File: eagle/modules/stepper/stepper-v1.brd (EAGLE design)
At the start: 100 x 80 mm, 11 parts, among them J1 RJ12RIGHTANGLE

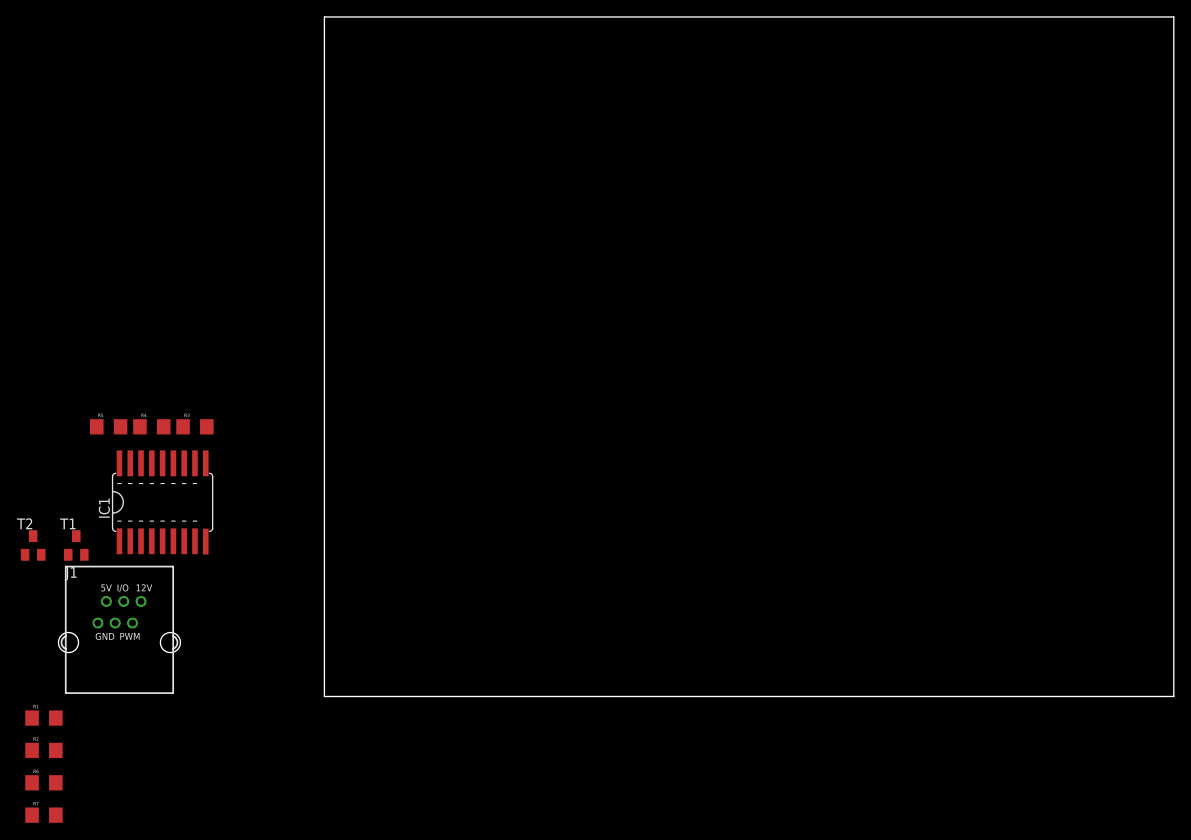
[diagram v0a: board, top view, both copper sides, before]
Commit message: Update Stepper
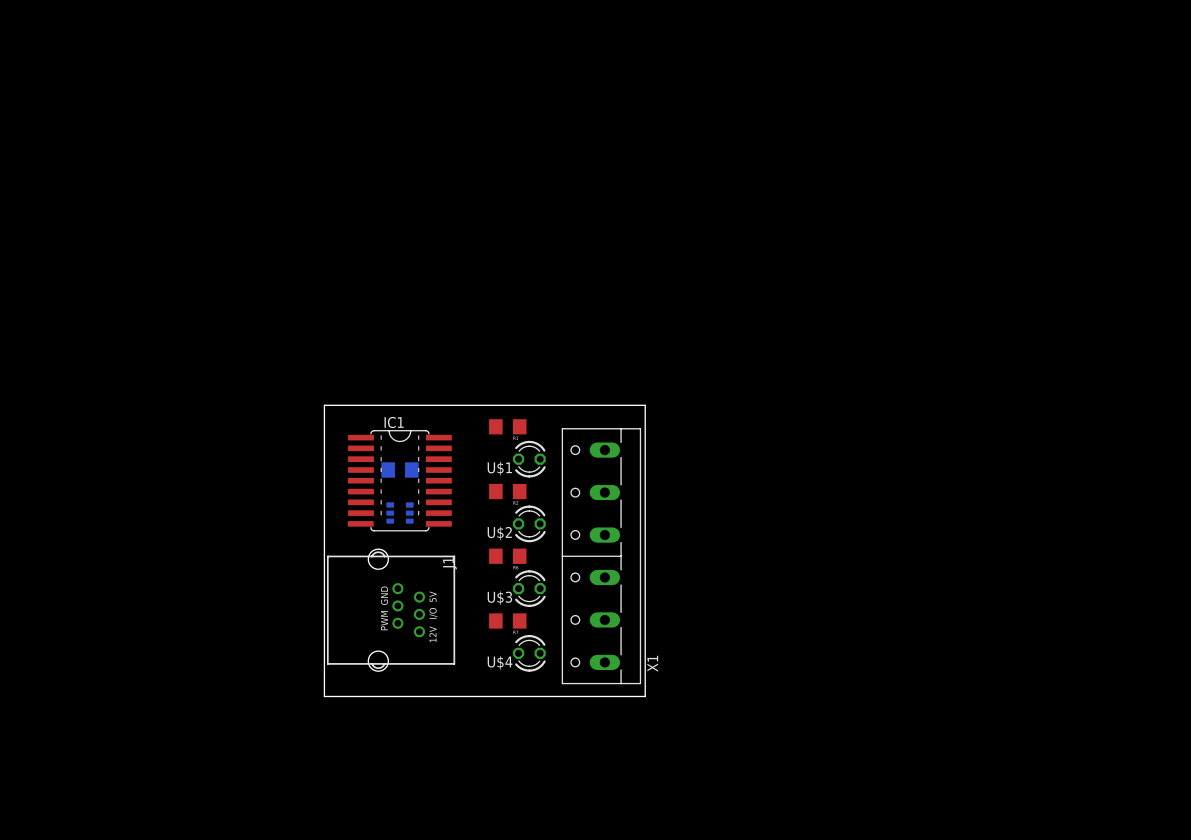
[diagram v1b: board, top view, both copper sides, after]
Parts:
- removed R3, R4: 1k, SparkFun:1206
- removed T1, T2: (no value), transistor:SOT23-BEC
- added IC2: SN74LVC2G14, lpatiny:SOT23-6
- added U$1, U$2, U$3, U$4: LED3MM, lpatiny:LED3MM
- added X1: (no value), con-wago-500:W237-6
- moved R1 64.5 mm to (21.6, 31.8), turned to 180 degrees
- moved R2 62.5 mm to (21.6, 24.1), turned to 180 degrees
- moved R6 60.8 mm to (21.6, 16.5), turned to 180 degrees
- moved R7 59.2 mm to (21.6, 8.89), turned to 180 degrees
- moved R5 34.7 mm to (8.89, 26.7), flipped to the bottom, turned to 180 degrees
- moved J1 30.7 mm to (6.35, 10.2), turned to 270 degrees
- moved IC1 28.1 mm to (8.89, 25.4), turned to 270 degrees
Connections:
- removed net N$15: IC1.7, IC1.8, R4.2, T2.C
- new net N$10: R2.1, U$2.K
- new net N$11: R6.1, U$3.K
- new net N$12: R7.1, U$4.K
- new net N$7: IC1.7, IC1.8, IC2.4
- new net N$9: R1.1, U$1.K
- net +12V: now also X1.2, X1.5
- net +5V: now also IC2.5, U$1.A, U$2.A, U$3.A, U$4.A; no longer R3.1, R4.1
- net GND: now also IC2.2; no longer T1.E, T2.E
- net N$1: now also IC2.1; no longer T1.B
- net N$14: now also IC1.5, IC1.6, IC2.6; no longer IC1.3, IC1.4, R3.2, T1.C
- net N$2: now also IC1.3, IC1.4, IC2.3; no longer IC1.5, IC1.6, T2.B
- net N$3: now also X1.6
- net N$4: now also X1.4
- net N$5: now also X1.3
- net N$6: now also X1.1
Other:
- board size 100 x 80 mm -> 37.8 x 34.3 mm
- board text added: "Stepper 1.0 - 12V"
